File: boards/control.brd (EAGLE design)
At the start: 100 x 80 mm, 53 parts, among them IC1 MEGA16-P, IC2 7805TV, Q2 BS250, Q3 IRF530, Q4 IRF530, Q5 IRF530, Q6 IRF530, X1 USBPTH

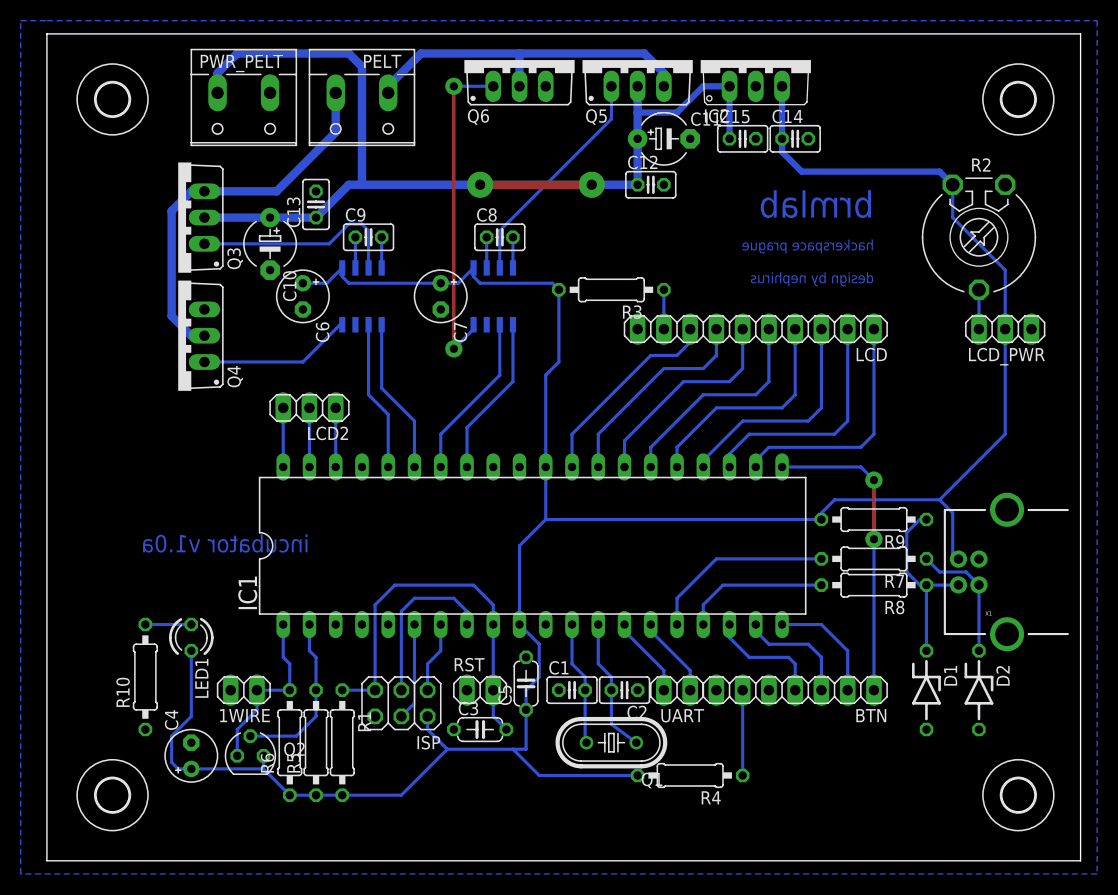
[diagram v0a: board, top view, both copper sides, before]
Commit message: put all the downloaded files into directories
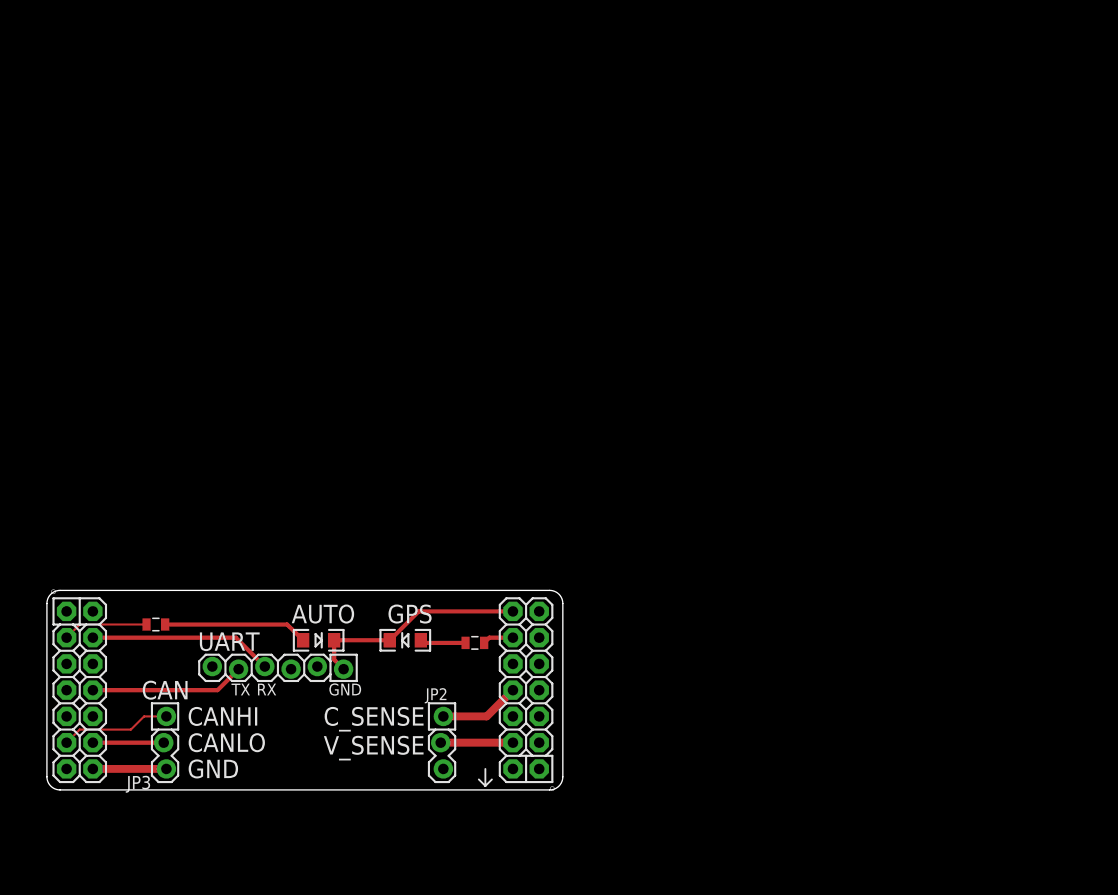
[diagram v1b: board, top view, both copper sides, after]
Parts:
- removed 1WIRE, RST, UART: (no value), pinhead:1X02
- removed BTN: (no value), pinhead:1X07
- removed C1, C2: (no value), resistor:C025-025X050
- removed C10, C11: 4u7, resistor:E5-5
- removed C12, C13, C14, C8, C9: 100n, resistor:C025-025X050
- removed C15: 330n, resistor:C025-025X050
- removed C3, C5: (no value), resistor:C050-024X044
- removed C4: (no value), resistor:E2,5-5
- removed C6, C7: 10u, resistor:E2,5-5
- removed D1, D2: 3V6, diode:ZDIO-7.5
- removed H1, H2, H3, H4: MOUNT-HOLE3.2, holes:3,2
- removed IC1: MEGA16-P, atmel:DIL40
- removed IC2: 7805TV, linear:TO220V
- removed ISP: (no value), pinhead:2X03
- removed LCD: (no value), pinhead:1X10
- removed LCD2, LCD_PWR: (no value), pinhead:1X03
- removed PELT, PWR_PELT: (no value), con-wago-508:W237-132
- removed Q1: (no value), crystal:HC49U-V
- removed Q2: BS250, transistor-small-signal:SOT54E
- removed Q3, Q4, Q5, Q6: IRF530, transistor-power:TO220BV
- removed R10: 270R, resistor:0207/10
- removed R3, R4, R5: ??, resistor:0207/10
- removed R6: 4k7, resistor:0207/10
- removed R7, R8: 68R, resistor:0207/10
- removed R9: 1k5, resistor:0207/10
- removed U$2: LM5101, lm5101:SOIC8
- removed X1: USBPTH, SparkFun:USB-B-PTH
- added JP1: (no value), ASL:1X06_LOCK
- added JP2, JP3: M03LOCK, ASL:1X03_LOCK
- added LED2: (no value), ASL:LED-1206
- LED1: device led:LED3MM -> ASL:LED-1206
- R1: value 4k7 -> 330; device resistor:0207/10 -> ASL:0805
- R2: value (none) -> 330; device pot:LI10 -> ASL:0805
- U$1: value LM5101 -> CANODE_SHIELD; device lm5101:SOIC8 -> ASL:CANODE_SHIELD
- moved R2 88.0 mm to (10.5, 22.9)
- moved U$1 62.5 mm to (0.00, 0.00), flipped to the top, turned to 0 degrees
- moved LED1 20.7 mm to (34.7, 21.3), turned to 180 degrees
- moved R1 16.1 mm to (41.4, 21.1), turned to 0 degrees
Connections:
- removed net +5V: C14.1, C4.+, C5.1, C6.+, C7.+, IC1.10, IC1.30, IC2.3, ISP.2, LCD_PWR.2, LED1.K, Q2.S, R1.2, R2.E, R3.2, R4.2, R5.1, R6.1, R9.2, U$1.1, U$2.1, X1.VBUS
- removed net GND: 1WIRE.2, BTN.5, BTN.7, C1.1, C10.-, C11.-, C12.2, C13.2, C14.2, C15.2, C2.1, C3.1, C4.-, C5.2, C6.-, C7.-, D1.A, D2.A, IC1.11, IC1.31, IC2.2, ISP.6, LCD.10, LCD_PWR.1, PWR_PELT.1, Q4.S, Q6.S, R10.1, R2.A, RST.1, U$1.7, U$2.7, X1.GND
- removed net MISO: IC1.7, ISP.1
- removed net MOSI: IC1.6, ISP.4
- removed net N$10: IC1.25, LCD.4
- removed net N$11: IC1.26, LCD.5
- removed net N$12: IC1.27, LCD.6
- removed net N$13: IC1.28, LCD.7
- removed net N$14: IC1.29, LCD.8
- removed net N$15: IC1.40, LCD2.3
- removed net N$16: IC1.39, LCD2.2
- removed net N$17: IC1.38, LCD2.1
- removed net N$18: IC1.16, R7.2
- removed net N$19: IC1.17, R8.2
- removed net N$20: BTN.6, R4.1
- removed net N$21: BTN.1, IC1.21
- removed net N$22: BTN.2, IC1.20
- removed net N$23: BTN.3, IC1.19
- removed net N$24: BTN.4, IC1.18
- removed net N$25: 1WIRE.1, IC1.1, Q2.D, R6.2
- removed net N$26: IC1.15, UART.1
- removed net N$27: IC1.14, UART.2
- removed net N$28: D2.C, R7.1, X1.D+
- removed net N$29: D1.C, R8.1, R9.1, X1.D-
- removed net N$3: IC1.33, U$2.5
- removed net N$30: IC1.34, U$2.6
- removed net N$31: IC1.35, U$1.5
- removed net N$32: IC1.36, U$1.6
- removed net N$33: C9.1, U$1.2
- removed net N$34: C8.1, U$2.2
- removed net N$35: C8.2, U$2.4
- removed net N$36: C9.2, U$1.4
- removed net N$37: PELT.2, Q3.S, Q4.D
- removed net N$38: PELT.1, Q5.S, Q6.D
- removed net N$39: Q3.G, U$1.3
- removed net N$4: IC1.2, Q2.G, R5.2
- removed net N$40: Q4.G, U$1.8
- removed net N$41: Q5.G, U$2.3
- removed net N$42: Q6.G, U$2.8
- removed net N$43: LED1.A, R10.2
- removed net N$46: C10.+, C11.+, C12.1, C13.1, C15.1, IC2.1, PWR_PELT.2, Q3.D, Q5.D
- removed net N$5: LCD.9, R3.1
- removed net N$6: LCD_PWR.3, R2.S
- removed net N$7: IC1.22, LCD.1
- removed net N$8: IC1.23, LCD.2
- removed net N$9: IC1.24, LCD.3
- removed net RESET: C3.2, IC1.9, ISP.5, R1.1, RST.2
- removed net SCK: IC1.8, ISP.3
- new net CAN_HI: JP3.1, U$1.CAN_HIGH
- new net CAN_LO: JP3.2, U$1.CAN_LOW
- new net CURRENT_SENSE: JP2.1, U$1.RB1
- new net GND2: JP1.1, LED1.C, LED2.C, U$1.GND
- new net GND3: U$1.GND7
- new net GND4: JP3.3, U$1.GND4
- new net LED_AUTOMODE: R2.2, U$1.RB12
- new net LED_GPS: R1.2, U$1.RB15
- new net UART_RX: JP1.4, U$1.RB9
- new net UART_TX: JP1.5, U$1.RB8
- new net VOLTAGE_SENSE: JP2.2, U$1.A0
- net N$1: now also LED1.A, R1.1; no longer C1.2, IC1.12, Q1.2
- net N$2: now also LED2.A, R2.1; no longer C2.2, IC1.13, Q1.1
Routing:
- net +5V: track 248.3 -> 0.00 mm
- net N$46: track 96.4 -> 0.00 mm, vias 2 -> 0
- net RESET: track 37.0 -> 0.00 mm
- net N$37: track 37.0 -> 0.00 mm
- net N$38: track 33.9 -> 0.00 mm
- net N$42: track 32.3 -> 0.00 mm, vias 2 -> 0
- net N$21: track 29.7 -> 0.00 mm, vias 2 -> 0
- net N$7: track 23.3 -> 0.00 mm
- net N$8: track 22.9 -> 0.00 mm
- net N$41: track 22.0 -> 0.00 mm
- net N$9: track 21.8 -> 0.00 mm
- net N$10: track 21.8 -> 0.00 mm
- net GND2: track 0.00 -> 21.6 mm
- net N$11: track 21.0 -> 0.00 mm
- net N$12: track 20.7 -> 0.00 mm
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- removed copper zone on layer 16, net GND
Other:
- board size 100 x 80 mm -> 49.9 x 19.3 mm
- board text added: "AUTO"
- board text added: "CAN"
- board text added: "CANHI"
- board text added: "CANLO"
- board text added: "C_SENSE"
- board text added: "GND"
- board text added: "GPS"
- board text added: "RX"
- board text added: "TX"
- board text added: "UART"
- board text added: "V_SENSE"
- board text removed: "brmlab"
- board text removed: "design by nephirus"
- board text removed: "hackerspace prague"
- board text removed: "incubator v1.0a"
